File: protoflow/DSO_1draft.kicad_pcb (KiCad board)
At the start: 2 copper layers, 99.9 x 77.2 mm, 130 parts, among them J1 Conn_01x05, J2 Conn_Coaxial, J3 Conn_Coaxial, J4 Conn_Coaxial, J5 Conn_Coaxial, J7 USB_A_Stacked, J8 Conn_01x20, J9 Conn_01x20, SW1 SW_SPDT, SW2 SW_SPDT, SW3 SW_SPDT, SW4 SW_SPDT, SW5 SW_SPDT, U1 ADG708BRUZ, U2 ADG708BRUZ, U3 STM32G431C6Tx

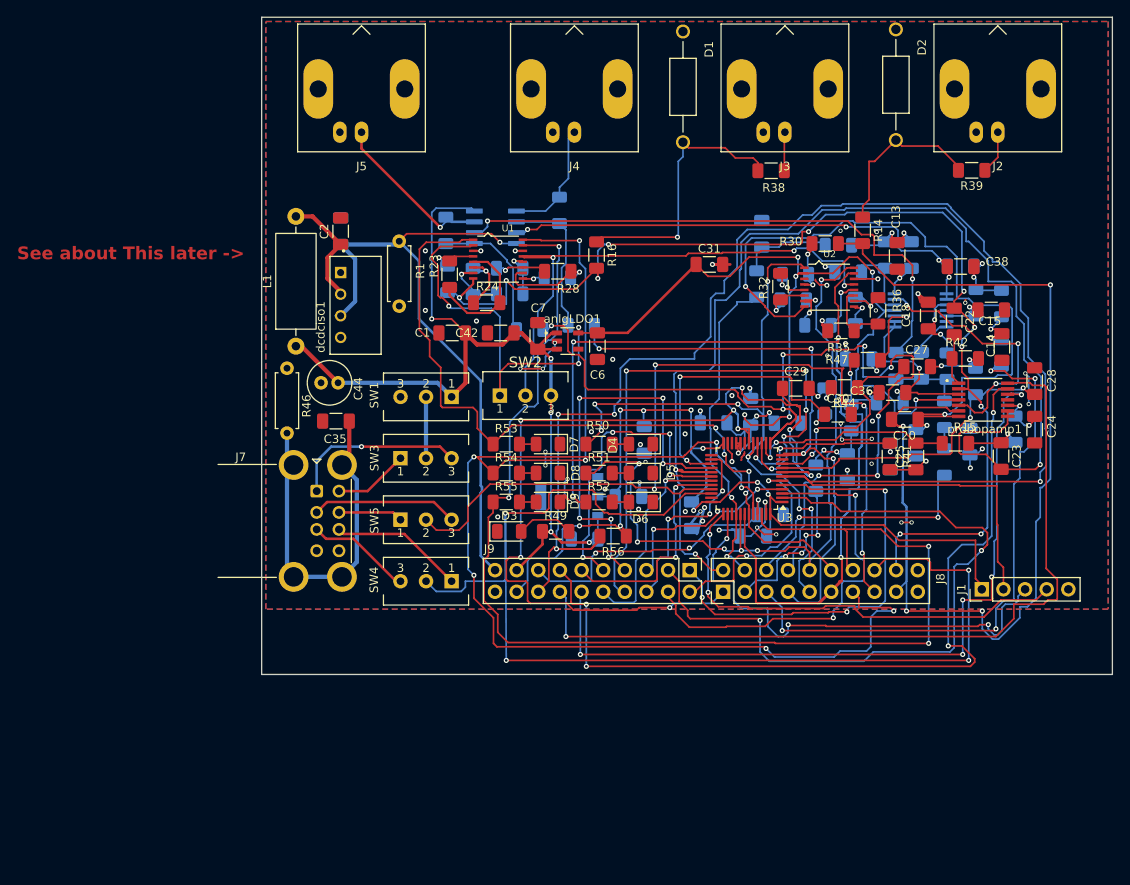
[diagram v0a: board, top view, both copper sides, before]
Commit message: all done
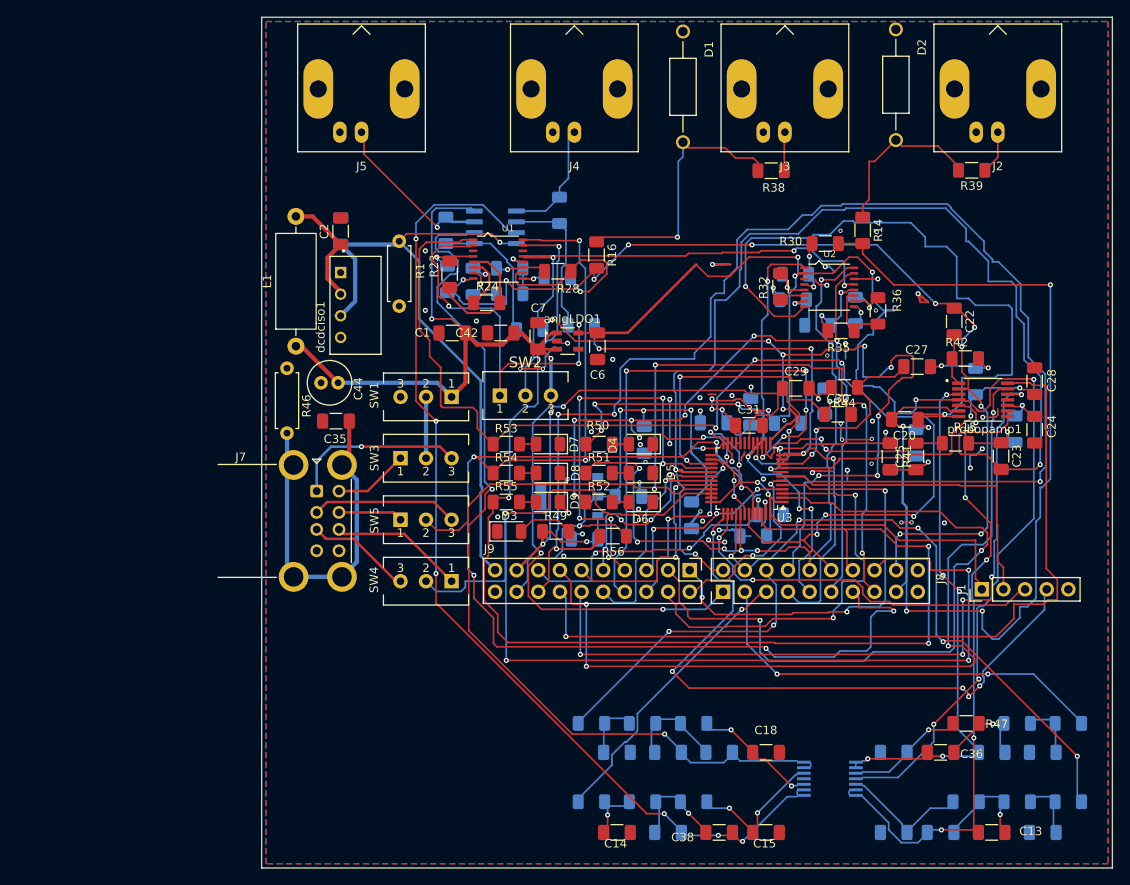
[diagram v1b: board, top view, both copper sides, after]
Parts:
- moved C11 77.7 mm to (175.0, 174.8), turned to 180 degrees
- moved C16 74.8 mm to (131.0, 174.8), turned to 0 degrees
- moved C14 72.7 mm to (125.0, 174.8), turned to 0 degrees
- moved C38 72.2 mm to (137.0, 174.8), turned to 0 degrees
- moved R9 72.1 mm to (128.0, 171.2), turned to 0 degrees
- moved R8 71.4 mm to (122.0, 171.2), turned to 0 degrees
- moved R5 71.0 mm to (178.0, 171.2), turned to 180 degrees
- moved R6 68.6 mm to (172.0, 171.2), turned to 180 degrees
- moved C13 68.6 mm to (169.0, 174.8), turned to 180 degrees
- moved C37 67.9 mm to (163.0, 174.8), turned to 180 degrees
- moved R10 67.3 mm to (134.0, 171.2), turned to 0 degrees
- moved C15 66.8 mm to (142.5, 174.8)
- moved C12 66.0 mm to (157.5, 174.8)
- moved R7 64.9 mm to (166.0, 171.2), turned to 180 degrees
- moved pwmoppamp1 56.0 mm to (150.0, 168.5), turned to 180 degrees
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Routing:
- net /3v3: track 167.5 -> 229.7 mm, vias 12 -> 14
- net /B2: track 164.3 -> 105.6 mm, vias 4 -> 11
- net /pwmout3: track 60.8 -> 111.9 mm, vias 4 -> 6
- net /A0: track 89.2 -> 137.8 mm, vias 4 -> 6
- net /PB3_TM2_3: track 69.7 -> 32.4 mm, vias 4 -> 1
- net /PA0_ADC_IN1: track 128.3 -> 94.1 mm, vias 8 -> 5
- net /pwmout1: track 22.0 -> 56.1 mm, vias 2 -> 5
- net /PB3_TM2_2: track 38.3 -> 69.4 mm, vias 2 -> 5
- net /pwmout2: track 38.3 -> 67.7 mm, vias 4 -> 5
- net /PB3_TM2_1: track 18.9 -> 47.6 mm, vias 4 -> 2
- net /pwmout4: track 75.2 -> 99.4 mm
- net /PA13_SWDIO: track 53.1 -> 74.8 mm, vias 2 -> 5
- net /S0: track 131.8 -> 117.5 mm
- net /PA8: track 36.8 -> 22.8 mm, vias 4 -> 3
- net /PA14_SCLK: track 56.6 -> 43.4 mm, vias 3 -> 2
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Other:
- board size 99.9 x 77.2 mm -> 99.9 x 99.9 mm

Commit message: Revert "all done"
This reverts commit f6672cdd42e4cabdd9d70339eddc16dd63b2a9c6.
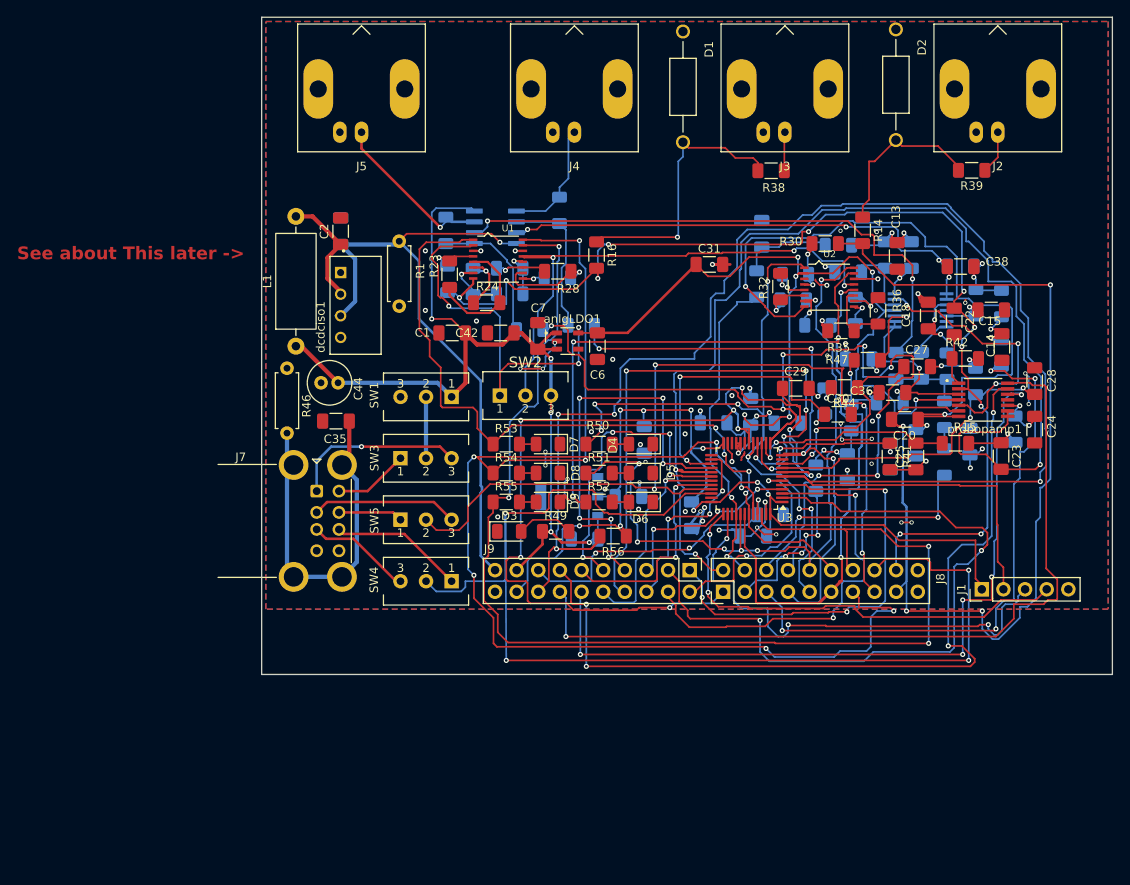
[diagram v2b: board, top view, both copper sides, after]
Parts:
- moved C11 77.7 mm to (142.0, 104.5), turned to 90 degrees
- moved C16 74.8 mm to (165.3, 108.3), turned to 180 degrees
- moved C14 72.7 mm to (170.2, 117.8), turned to -90 degrees
- moved C38 72.2 mm to (165.3, 108.3), turned to 180 degrees
- moved R9 72.1 mm to (170.2, 112.7), turned to 90 degrees
- moved R8 71.4 mm to (170.2, 118.5), turned to 90 degrees
- moved R5 71.0 mm to (141.4, 110.4), turned to 90 degrees
- moved R6 68.6 mm to (151.0, 105.8), turned to 0 degrees
- moved C13 68.6 mm to (157.9, 107.1), turned to -90 degrees
- moved C37 67.9 mm to (159.6, 107.0), turned to -90 degrees
- moved R10 67.3 mm to (167.2, 112.6), turned to -90 degrees
- moved C15 66.8 mm to (168.9, 113.5)
- moved C12 66.0 mm to (152.2, 109.0)
- moved R7 64.9 mm to (156.5, 107.0), turned to -90 degrees
- moved pwmoppamp1 56.0 mm to (160.7, 113.5), turned to 0 degrees
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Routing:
- net /3v3: track 229.7 -> 167.5 mm, vias 14 -> 12
- net /B2: track 105.6 -> 164.3 mm, vias 11 -> 4
- net /pwmout3: track 111.9 -> 60.8 mm, vias 6 -> 4
- net /A0: track 137.8 -> 89.2 mm, vias 6 -> 4
- net /PB3_TM2_3: track 32.4 -> 69.7 mm, vias 1 -> 4
- net /PA0_ADC_IN1: track 94.1 -> 128.3 mm, vias 5 -> 8
- net /pwmout1: track 56.1 -> 22.0 mm, vias 5 -> 2
- net /PB3_TM2_2: track 69.4 -> 38.3 mm, vias 5 -> 2
- net /pwmout2: track 67.7 -> 38.3 mm, vias 5 -> 4
- net /PB3_TM2_1: track 47.6 -> 18.9 mm, vias 2 -> 4
- net /pwmout4: track 99.4 -> 75.2 mm
- net /PA13_SWDIO: track 74.8 -> 53.1 mm, vias 5 -> 2
- net /S0: track 117.5 -> 131.8 mm
- net /PA8: track 22.8 -> 36.8 mm, vias 3 -> 4
- net /PA14_SCLK: track 43.4 -> 56.6 mm, vias 2 -> 3
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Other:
- board size 99.9 x 99.9 mm -> 99.9 x 77.2 mm
